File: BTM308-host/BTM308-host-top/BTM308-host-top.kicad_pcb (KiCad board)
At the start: 4 copper layers, 52.8 x 40.1 mm, 52 parts, among them J1 Bottom, J2 USB_C_Receptacle_USB2.0_16P, J3 Battery +, J4 Battery -, J5 Top, J6 Battery +, J7 Battery -, SW1 PLAY, SW2 VOL-, SW3 VOL+, SW4 ON/OFF, SW6 Battery Status, U1 Bluetooth Module, U2 OPA1678, U3 PJ-320A

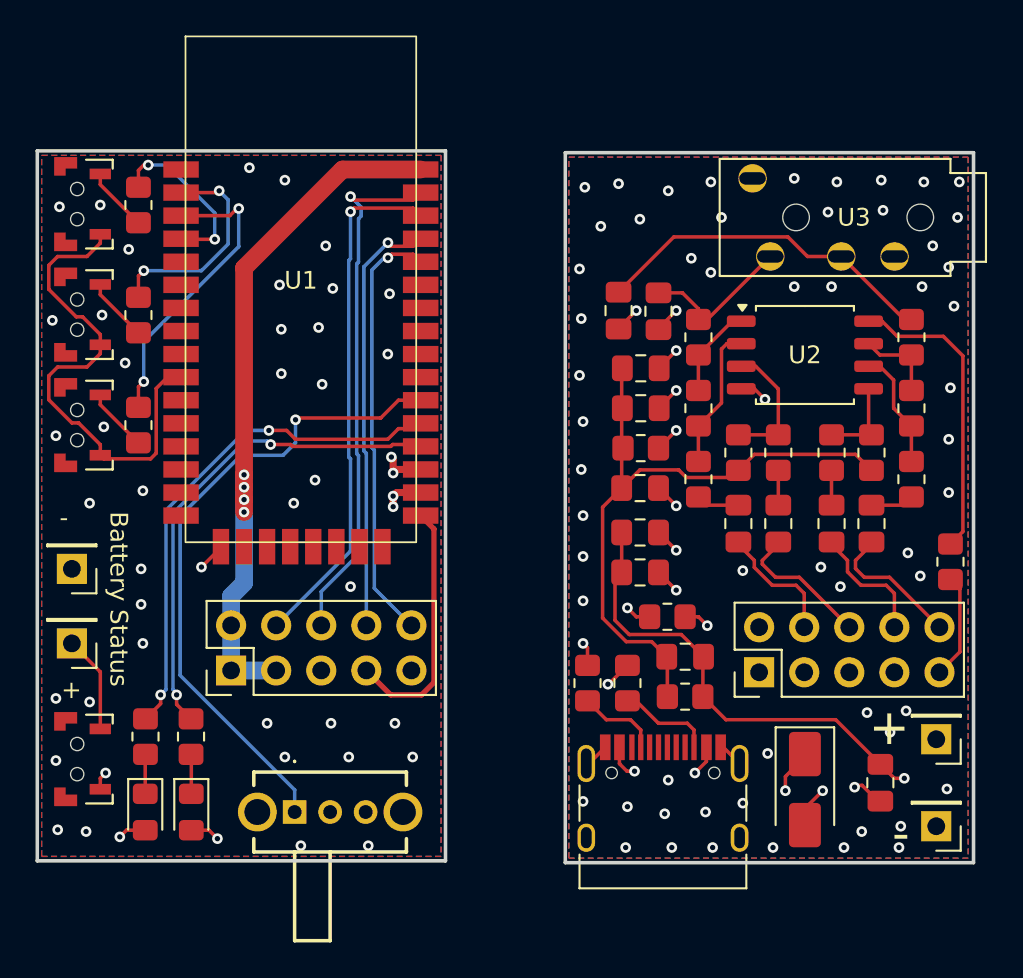
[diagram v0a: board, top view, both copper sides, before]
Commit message: fab
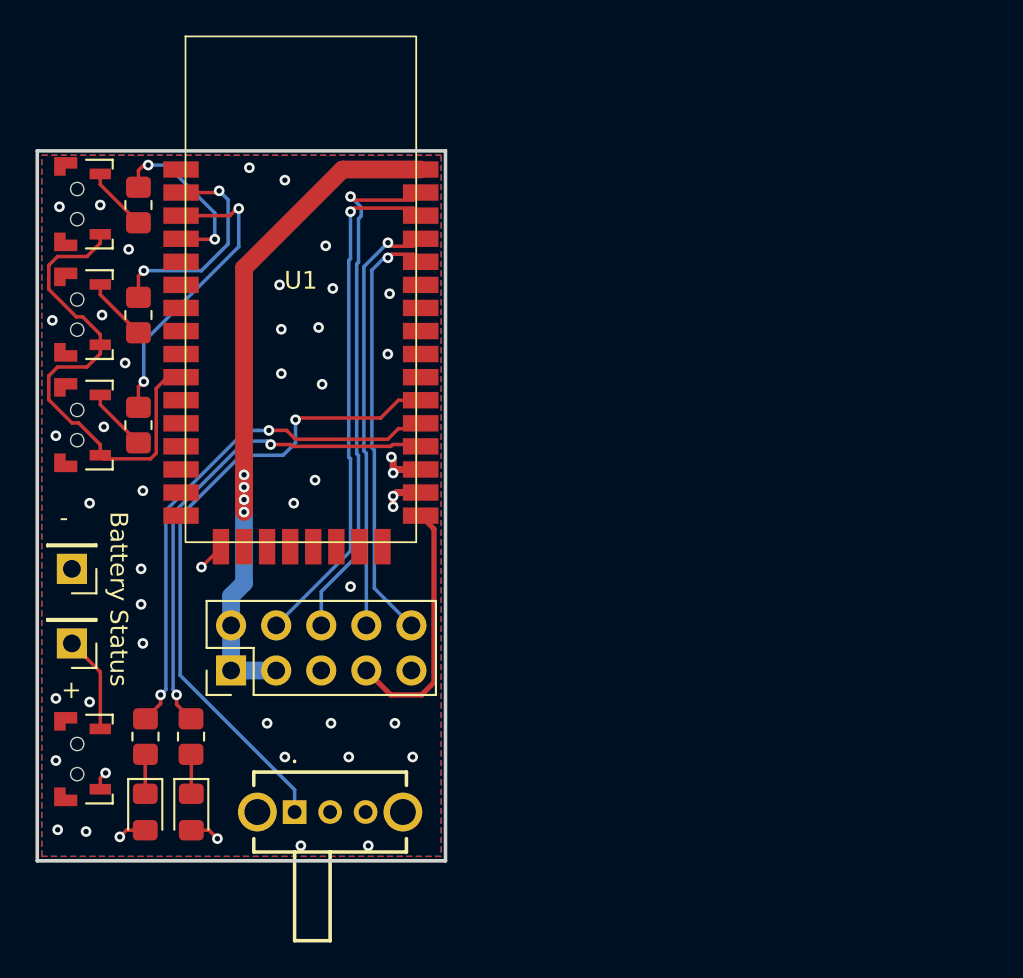
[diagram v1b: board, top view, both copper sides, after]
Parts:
- removed C1, C11, C2: 220uF, Capacitor_SMD:C_0805_2012Metric_Pad1.18x1.45mm_HandSolder
- removed C10, C3, C5: 22uF, Capacitor_SMD:C_0805_2012Metric_Pad1.18x1.45mm_HandSolder
- removed C12, C13: 10uf, Capacitor_SMD:C_0805_2012Metric_Pad1.18x1.45mm_HandSolder
- removed C4: 100nF, Capacitor_SMD:C_0805_2012Metric_Pad1.18x1.45mm_HandSolder
- removed C6, C7, C8, C9: 1uF, Capacitor_SMD:C_0805_2012Metric_Pad1.18x1.45mm_HandSolder
- removed D3: SMAJ6.0A, Diode_SMD:D_SMA
- removed J1: Bottom, Connector_PinHeader_2.54mm:PinHeader_2x05_P2.54mm_Vertical
- removed J2: USB_C_Receptacle_USB2.0_16P, Connector_USB:USB_C_Receptacle_HRO_TYPE-C-31-M-12
- removed J3: Battery +, Connector_PinHeader_2.54mm:PinHeader_1x01_P2.54mm_Vertical
- removed J4: Battery -, Connector_PinHeader_2.54mm:PinHeader_1x01_P2.54mm_Vertical
- removed R10, R11, R12, R13, R15, R16, R6, R7, R8, R9: 10k, Resistor_SMD:R_0805_2012Metric_Pad1.20x1.40mm_HandSolder
- removed R14, R21: 0, Resistor_SMD:R_0805_2012Metric_Pad1.20x1.40mm_HandSolder
- removed R17, R18: 5.1k, Resistor_SMD:R_0805_2012Metric_Pad1.20x1.40mm_HandSolder
- removed R19, R20: 47, Resistor_SMD:R_0805_2012Metric_Pad1.20x1.40mm_HandSolder
- removed U2: OPA1678, Package_SO:SOIC-8_5.3x5.3mm_P1.27mm
- removed U3: PJ-320A, PJ-320A_Library:PJ-320A
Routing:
- net /VREF: track 36.9 -> 0.00 mm
- net /VBAT: track 39.3 -> 6.87 mm, vias 6 -> 5
- net Net-(U3-Ring1): track 19.7 -> 0.00 mm
- net Net-(U2C-V+): track 17.0 -> 0.00 mm
- net AGND: track 54.3 -> 39.9 mm, vias 14 -> 4
- net GND: track 15.3 -> 3.84 mm, vias 106 -> 43
- net Net-(U3-Tip): track 8.74 -> 0.00 mm
- net Net-(U2A--): track 8.11 -> 0.00 mm
- net /SPK_AP: track 37.6 -> 29.6 mm
- net /SPK_BN: track 32.2 -> 24.2 mm
- net Net-(U2A-+): track 7.46 -> 0.00 mm
- net /SPK_AN: track 36.5 -> 29.3 mm
- net /SPK_BP: track 31.4 -> 24.3 mm
- net Net-(U2B--): track 6.73 -> 0.00 mm
- net /VCHG: track 20.6 -> 14.4 mm, vias 3 -> 0
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- removed copper zone on In2.Cu, net /VCHG
- removed copper zone on In1.Cu, net AGND
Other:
- board size 52.8 x 40.1 mm -> 23 x 40 mm
